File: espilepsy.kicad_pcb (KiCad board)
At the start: 2 copper layers, 42.2 x 53.2 mm, 33 parts, among them J1 Conn_01x06, J2 Screw_Terminal_01x02, J3 Screw_Terminal_01x02, J4 Screw_Terminal_01x02, J5 Screw_Terminal_01x02, Q1 BSS138, Q2 IRF9310, SW1 SW_Push, U1 NCP1117-3.3_SOT223, U2 74AHCT1G125, U3 ESP32-WROOM-32D, U4 74AHCT1G125

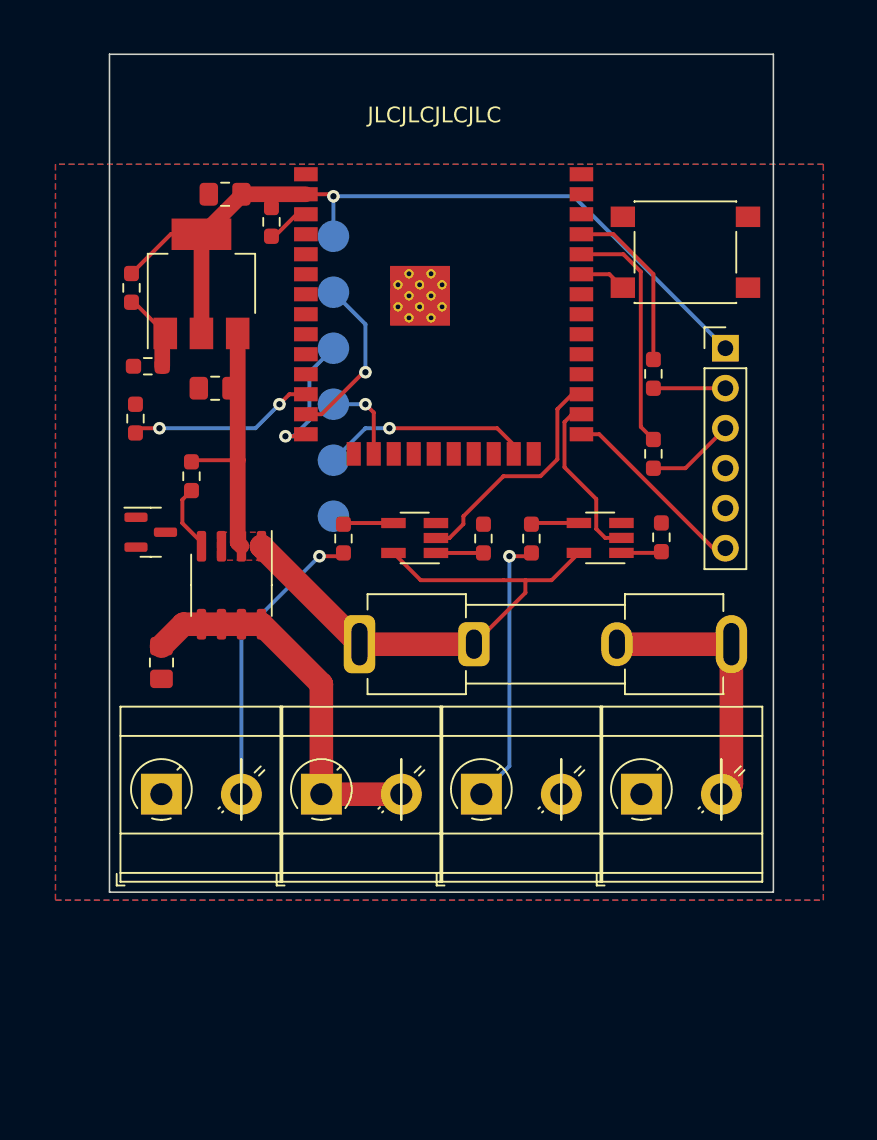
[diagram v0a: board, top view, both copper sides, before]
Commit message: Build v1
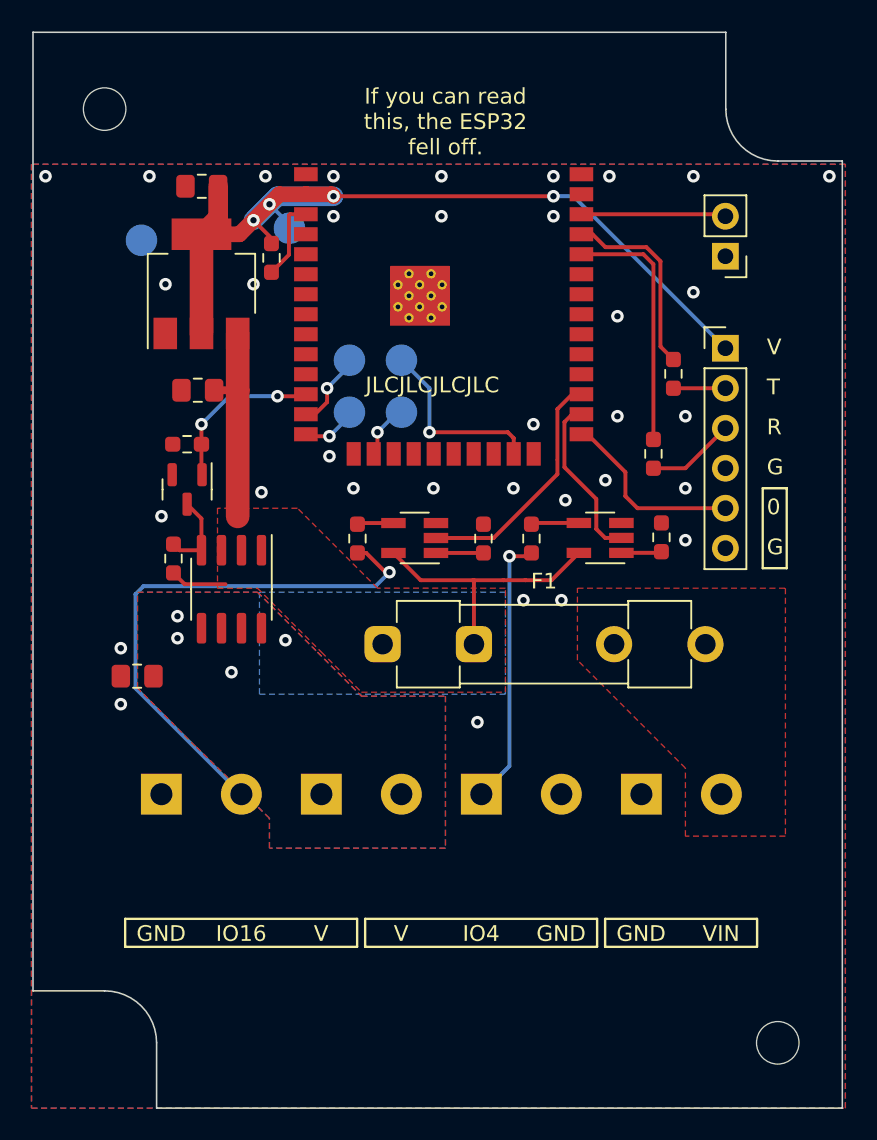
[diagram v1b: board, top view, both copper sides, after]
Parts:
- removed R2: R, Resistor_SMD:R_0603_1608Metric_Pad0.98x0.95mm_HandSolder
- removed R3: 0, Resistor_SMD:R_0603_1608Metric_Pad0.98x0.95mm_HandSolder
- removed SW1: SW_Push, Button_Switch_SMD:SW_Push_1P1T_NO_6x6mm_H9.5mm
- added H1: MountingHole, MountingHole:MountingHole_2.7mm_M2.5, F.Cu at (51.0, 53.9)
- added H2: MountingHole, MountingHole:MountingHole_2.7mm_M2.5, F.Cu at (93.8, 113.2)
- added J6: Conn_01x02_Pin, Connector_PinHeader_2.54mm:PinHeader_1x02_P2.54mm_Vertical, F.Cu at (90.4, 63.2)
- F1: footprint Fuse:Fuseholder_Clip-5x20mm_Keystone_3512P_Inline_P23.62x7.27mm_D1.02x2.41x1.02x1.57mm_Horizontal -> Fuse:Fuseholder_Clip-5x20mm_Littelfuse_520_Inline_P20.50x5.80mm_D1.30mm_Horizontal
- J2, J3, J4, J5: footprint TerminalBlock_MetzConnect:TerminalBlock_MetzConnect_Type073_RT02602HBLU_1x02_P5.08mm_Horizontal -> Library:TerminalBlock_MetzConnect_Type073_RT02602HBLU_1x02_P5.08mm_Horizontal_mod
- U2, U4: value 74AHCT1G125 -> M74VHC1GT50
- moved TP6 21.3 mm to (53.3, 62.2)
- moved TP5 7.68 mm to (69.8, 69.8)
- moved R5 5.35 mm to (55.4, 82.4), turned to 90 degrees
- moved TP2 4.44 mm to (66.5, 69.8)
- moved TP4 4.35 mm to (69.8, 73.2)
- moved TP3 4.19 mm to (66.5, 73.2)
- moved R4 3.66 mm to (56.2, 75.2), turned to 180 degrees
- moved Q1 3.57 mm to (56.2, 78.1), turned to -90 degrees
- moved TP1 2.84 mm to (62.7, 61.5)
- moved R1 2.29 mm to (61.6, 63.3)
- moved C3 1.77 mm to (53.1, 89.9), turned to 180 degrees
- moved C1 1.57 mm to (57.2, 58.8)
- moved F1 1.47 mm to (68.7, 87.9)
- moved R11 1.27 mm to (87.1, 70.7)
- moved C2 1.11 mm to (56.9, 71.8)
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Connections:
- net Net-(J5-Pin_2) renamed /VIN
- J1 pad 5: GND -> /IO0
- J1 pad 6: /IO0 -> GND
- U1 pad 1: Net-(U1-ADJ) -> GND
- U3 pad 33: /BTN_1 -> unconnected-(U3-IO21-Pad33)
- U3 pad 36: /IO22 -> /BTN_1
- U3 pad 37: /IO23 -> unconnected-(U3-IO23-Pad37)
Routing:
- net /LED_5V: track 24.4 -> 0.00 mm, vias 0 -> 4
- net +5V: track 51.3 -> 34.0 mm
- net /VIN: track 17.1 -> 0.00 mm
- net /LED_DATA_0_OUT: track 18.8 -> 34.7 mm
- net /BTN_1: track 2.98 -> 9.20 mm
- net /TMS: track 10.8 -> 4.92 mm
- net +3.3V: track 52.7 -> 57.9 mm, vias 1 -> 4
- net Net-(U1-ADJ): track 5.13 -> 0.00 mm
- net /TDI: track 8.50 -> 3.60 mm
- net /EN: track 2.76 -> 5.17 mm
- net /TCK: track 5.40 -> 3.52 mm
- net /TDO: track 13.3 -> 11.8 mm
- net Net-(U3-TXD0/IO1): track 11.0 -> 12.3 mm
- net /UART_TX: track 4.57 -> 3.30 mm
- net /LED_POWER: track 11.8 -> 10.6 mm
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- added copper zone on B.Cu, net +5V
- added copper zone on B.Cu, net /LED_5V
- added copper zone on F.Cu, net /LED_5V
- added copper zone on F.Cu, net /VIN
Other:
- board size 42.2 x 53.2 mm -> 51.4 x 68.3 mm
- board text added: "0"
- board text added: "ESPilepsy"
- board text added: "G"
- board text added: "GND"
- board text added: "IO16"
- board text added: "IO4"
- board text added: "If you can read this, the ESP32 fell off."
- board text added: "R"
- board text added: "T"
- board text added: "TCK"
- board text added: "TDI"
- board text added: "TDO"
- board text added: "TMS"
- board text added: "V"
- board text added: "VIN"
- board text added: "v1"
